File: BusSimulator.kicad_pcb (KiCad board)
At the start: 2 copper layers, 101.6 x 53.3 mm, 17 parts, among them J1 CONN_3-6318491-6, J2 CONN_3-6318491-6, U1 MPM3620, U2 MPM3620

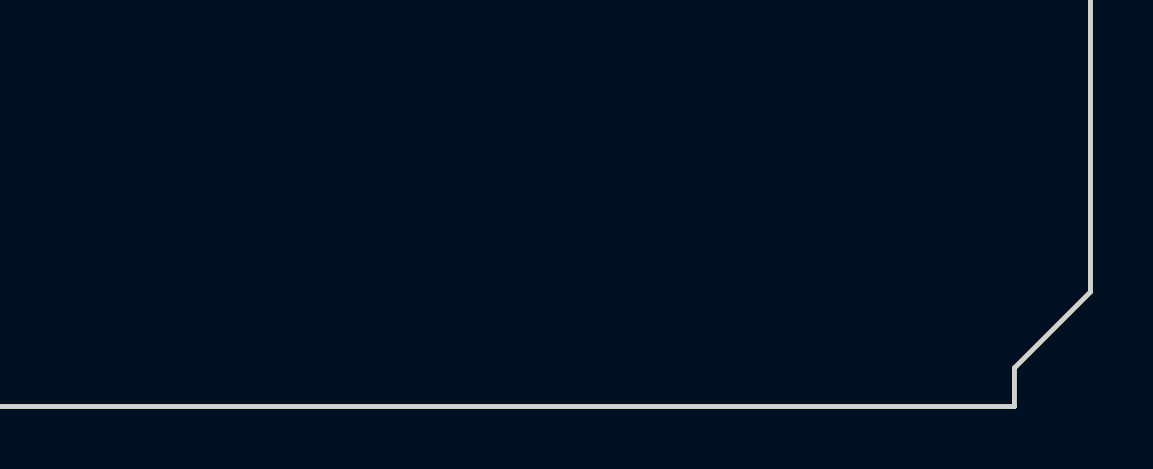
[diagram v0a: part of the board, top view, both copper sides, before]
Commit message: logo
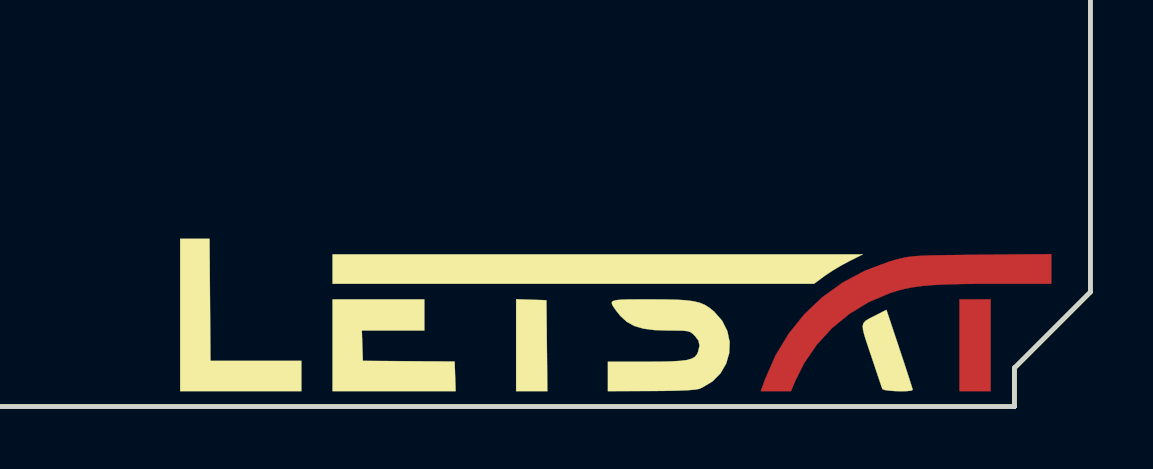
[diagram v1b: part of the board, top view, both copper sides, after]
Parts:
- added G1: LOGO, BusSimulator:LetSatLogo440, F.Cu at (195.9, 138.8)
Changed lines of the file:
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@@
     (links 92)
     (no_connects 59)
-    (area 109.924999 88.174999 211.675001 141.675001)
+    (area 108.853572 86.26384 211.882401 142.04484)
     (thickness 1.6)
     (drawings 10)
     (tracks 170)
     (zones 0)
-    (modules 17)
+    (modules 18)
     (nets 204)
   )
@@
       (net 16 GNDREF))
   )
+  (module BusSimulator:LetSatLogo440 (layer F.Cu)
+    (at 195.925 138.775)
+    (fp_text reference G1 (at 0 0) (layer F.SilkS) hide
+      (effects (font (thickness 0.3)))
+    )
+    (fp_text value LOGO (at 0.75 0) (layer F.SilkS) hide
+      (effects (font (thickness 0.3)))
+    )
+    (fp_poly (pts (xy 14.374091 -1.27) (xy 12.524543 -1.27) (xy 11.86217 -1.267926) (xy 11.301042 -1.260868)
+      (xy 10.827009 -1.247571) (xy 10.425923 -1.226781) (xy 10.083634 -1.197245) (xy 9.785993 -1.157707)
+      (xy 9.51885 -1.106914) (xy 9.268056 -1.043611) (xy 9.019462 -0.966544) (xy 8.990302 -0.956718)
+      (xy 8.295805 -0.66214) (xy 7.651998 -0.271547) (xy 7.070416 0.204436) (xy 6.562591 0.755186)
+      (xy 6.140059 1.370077) (xy 5.86025 1.926575) (xy 5.697679 2.309091) (xy 4.690238 2.309091)
+      (xy 4.830611 1.922368) (xy 5.178079 1.127685) (xy 5.615969 0.40227) (xy 6.138743 -0.248783)
+      (xy 6.740859 -0.820381) (xy 7.416777 -1.307428) (xy 8.160957 -1.704832) (xy 8.967859 -2.007498)
+      (xy 9.166755 -2.064535) (xy 9.308939 -2.102348) (xy 9.437794 -2.133407) (xy 9.566419 -2.158498)
+      (xy 9.70791 -2.178408) (xy 9.875366 -2.193924) (xy 10.081885 -2.205834) (xy 10.340563 -2.214924)
+      (xy 10.6645 -2.221982) (xy 11.066791 -2.227793) (xy 11.560536 -2.233146) (xy 12.050568 -2.237818)
+      (xy 14.374091 -2.25951) (xy 14.374091 -1.27)) (layer F.Cu) (width 0.01))
+    (fp_poly (pts (xy 12.353636 2.309091) (xy 11.314545 2.309091) (xy 11.314545 -0.750455) (xy 12.353636 -0.750455)
+      (xy 12.353636 2.309091)) (layer F.Cu) (width 0.01))
+    (fp_poly (pts (xy 14.374091 -1.27) (xy 12.524543 -1.27) (xy 11.86217 -1.267926) (xy 11.301042 -1.260868)
+      (xy 10.827009 -1.247571) (xy 10.425923 -1.226781) (xy 10.083634 -1.197245) (xy 9.785993 -1.157707)
+      (xy 9.51885 -1.106914) (xy 9.268056 -1.043611) (xy 9.019462 -0.966544) (xy 8.990302 -0.956718)
+      (xy 8.295805 -0.66214) (xy 7.651998 -0.271547) (xy 7.070416 0.204436) (xy 6.562591 0.755186)
+      (xy 6.140059 1.370077) (xy 5.86025 1.926575) (xy 5.697679 2.309091) (xy 4.690238 2.309091)
+      (xy 4.830611 1.922368) (xy 5.178079 1.127685) (xy 5.615969 0.40227) (xy 6.138743 -0.248783)
+      (xy 6.740859 -0.820381) (xy 7.416777 -1.307428) (xy 8.160957 -1.704832) (xy 8.967859 -2.007498)
+      (xy 9.166755 -2.064535) (xy 9.308939 -2.102348) (xy 9.437794 -2.133407) (xy 9.566419 -2.158498)
+      (xy 9.70791 -2.178408) (xy 9.875366 -2.193924) (xy 10.081885 -2.205834) (xy 10.340563 -2.214924)
+      (xy 10.6645 -2.221982) (xy 11.066791 -2.227793) (xy 11.560536 -2.233146) (xy 12.050568 -2.237818)
+      (xy 14.374091 -2.25951) (xy 14.374091 -1.27)) (layer F.Mask) (width 0.01))
+    (fp_poly (pts (xy 12.353636 2.309091) (xy 11.314545 2.309091) (xy 11.314545 -0.750455) (xy 12.353636 -0.750455)
+      (xy 12.353636 2.309091)) (layer F.Mask) (width 0.01))
+    (fp_poly (pts (xy -13.667671 -0.736023) (xy -13.6525 1.298863) (xy -10.621777 1.298863) (xy -10.621819 2.309091)
+      (xy -14.662728 2.309091) (xy -14.662728 -2.770909) (xy -13.682841 -2.770909) (xy -13.667671 -0.736023)) (layer F.SilkS) (width 0.01))
+    (fp_poly (pts (xy -6.523182 0.288636) (xy -8.605859 0.288636) (xy -8.58918 0.79375) (xy -8.5725 1.298863)
+      (xy -7.042728 1.310372) (xy -5.512955 1.321881) (xy -5.496276 1.815486) (xy -5.479596 2.309091)
+      (xy -9.582728 2.309091) (xy -9.582728 -0.750455) (xy -6.523182 -0.750455) (xy -6.523182 0.288636)) (layer F.SilkS) (width 0.01))
+    (fp_poly (pts (xy -2.958523 -0.738271) (xy -2.453409 -0.721591) (xy -2.422629 2.309091) (xy -3.463637 2.309091)
+      (xy -3.463637 -0.75495) (xy -2.958523 -0.738271)) (layer F.SilkS) (width 0.01))
+    (fp_poly (pts (xy 1.497471 -0.74795) (xy 1.896073 -0.738379) (xy 2.21182 -0.718657) (xy 2.460978 -0.685701)
+      (xy 2.659811 -0.636426) (xy 2.824587 -0.567749) (xy 2.971569 -0.476584) (xy 3.117024 -0.359847)
+      (xy 3.13287 -0.345981) (xy 3.404018 -0.03861) (xy 3.57669 0.306077) (xy 3.654188 0.670892)
+      (xy 3.639817 1.038648) (xy 3.536881 1.392158) (xy 3.348682 1.714235) (xy 3.078525 1.987693)
+      (xy 2.729714 2.195344) (xy 2.637216 2.23254) (xy 2.50326 2.258125) (xy 2.256329 2.278267)
+      (xy 1.898779 2.292861) (xy 1.432966 2.3018) (xy 1.024659 2.304699) (xy -0.404091 2.309091)
+      (xy -0.404091 1.327727) (xy 0.867763 1.327727) (xy 1.349503 1.3253) (xy 1.729122 1.316392)
+      (xy 2.019884 1.298563) (xy 2.235053 1.26937) (xy 2.387891 1.226373) (xy 2.491662 1.16713)
+      (xy 2.559629 1.089201) (xy 2.598094 1.009261) (xy 2.650531 0.793553) (xy 2.612723 0.619426)
+      (xy 2.486713 0.457377) (xy 2.411758 0.386036) (xy 2.340291 0.338311) (xy 2.248207 0.309456)
+      (xy 2.111407 0.294723) (xy 1.905788 0.289366) (xy 1.629978 0.288636) (xy 1.158536 0.274068)
+      (xy 0.780369 0.225645) (xy 0.476448 0.136287) (xy 0.22774 -0.001086) (xy 0.015217 -0.193555)
+      (xy -0.120588 -0.362611) (xy -0.207648 -0.483916) (xy -0.26347 -0.576875) (xy -0.277165 -0.645255)
+      (xy -0.237846 -0.692828) (xy -0.134623 -0.723362) (xy 0.04339 -0.740626) (xy 0.307082 -0.74839)
+      (xy 0.667341 -0.750424) (xy 0.999749 -0.750455) (xy 1.497471 -0.74795)) (layer F.SilkS) (width 0.01))
+    (fp_poly (pts (xy 9.318607 0.910594) (xy 9.440983 1.27947) (xy 9.550148 1.611853) (xy 9.641061 1.892114)
+      (xy 9.708679 2.104624) (xy 9.747957 2.233755) (xy 9.755909 2.265821) (xy 9.703776 2.292592)
+      (xy 9.568413 2.30782) (xy 9.38137 2.312407) (xy 9.174199 2.307253) (xy 8.978452 2.293259)
+      (xy 8.825679 2.271325) (xy 8.747431 2.242352) (xy 8.743862 2.236931) (xy 8.717748 2.16153)
+      (xy 8.661322 1.995026) (xy 8.580788 1.755845) (xy 8.482351 1.462414) (xy 8.372213 1.133157)
+      (xy 8.369716 1.125681) (xy 8.24534 0.756685) (xy 8.155402 0.481075) (xy 8.102272 0.281322)
+      (xy 8.088322 0.1399) (xy 8.115925 0.039281) (xy 8.18745 -0.038061) (xy 8.30527 -0.109654)
+      (xy 8.471757 -0.193025) (xy 8.553721 -0.234215) (xy 8.881305 -0.401364) (xy 9.318607 0.910594)) (layer F.SilkS) (width 0.01))
+    (fp_poly (pts (xy 7.631314 -2.019188) (xy 7.363462 -1.874776) (xy 7.082892 -1.707016) (xy 6.844508 -1.548963)
+      (xy 6.816286 -1.528507) (xy 6.46513 -1.27) (xy -9.582728 -1.27) (xy -9.582728 -2.251364)
+      (xy 8.095187 -2.251364) (xy 7.631314 -2.019188)) (layer F.SilkS) (width 0.01))
+  )
   (gr_line (start 110 88.25) (end 207.525 88.25) (layer Edge.Cuts) (width 0.15))
